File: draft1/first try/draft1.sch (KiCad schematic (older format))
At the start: 2 parts

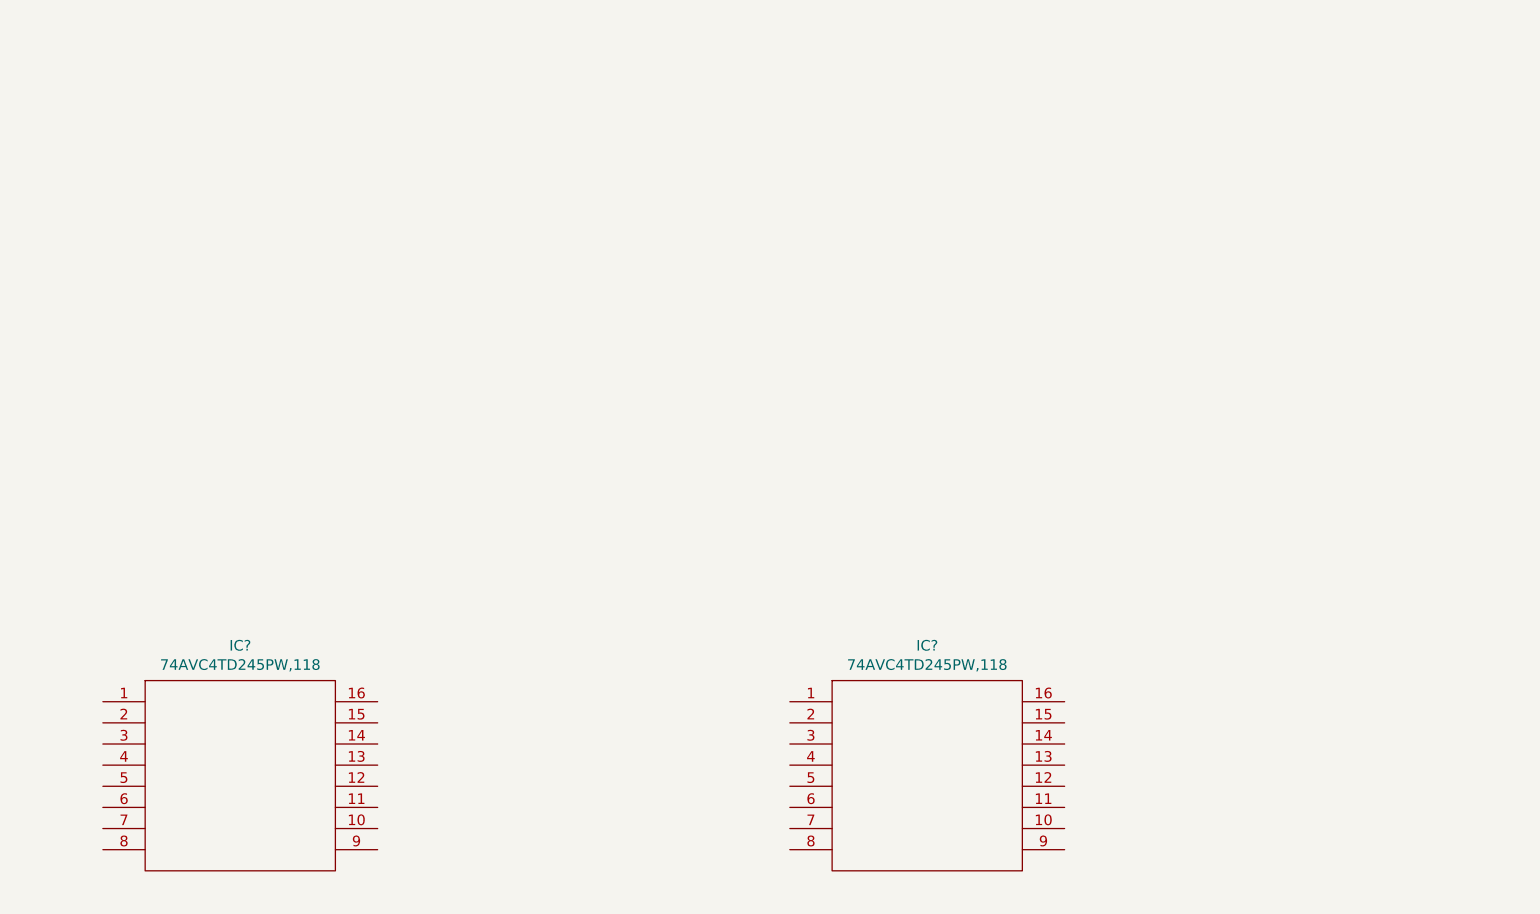
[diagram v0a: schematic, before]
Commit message: added connector
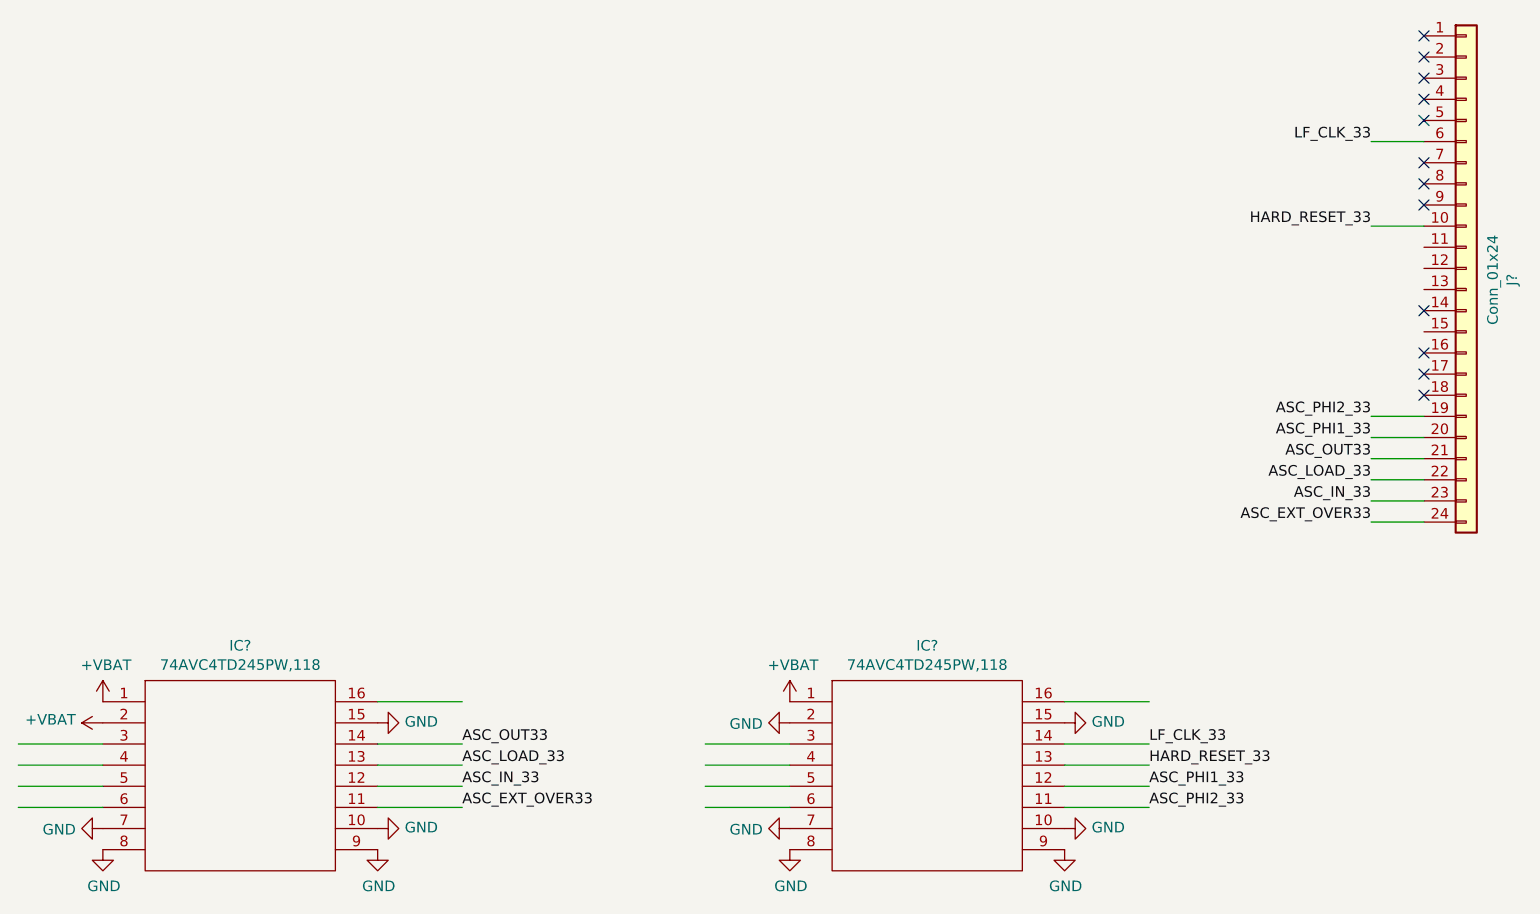
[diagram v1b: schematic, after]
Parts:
- added J?: Conn_01x24, symbol Connector_Generic:Conn_01x24
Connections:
- net labels added: +VBAT, ASC_EXT_OVER33, ASC_IN_33, ASC_LOAD_33, ASC_OUT33, ASC_PHI1_33, ASC_PHI2_33, GND, HARD_RESET_33, LF_CLK_33
- wire segments 0 -> 26
- no-connect marks 0 -> 12
